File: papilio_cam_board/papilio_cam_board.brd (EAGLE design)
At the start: 68.6 x 68.6 mm, 23 parts, among them U2 V_REG_317SMD

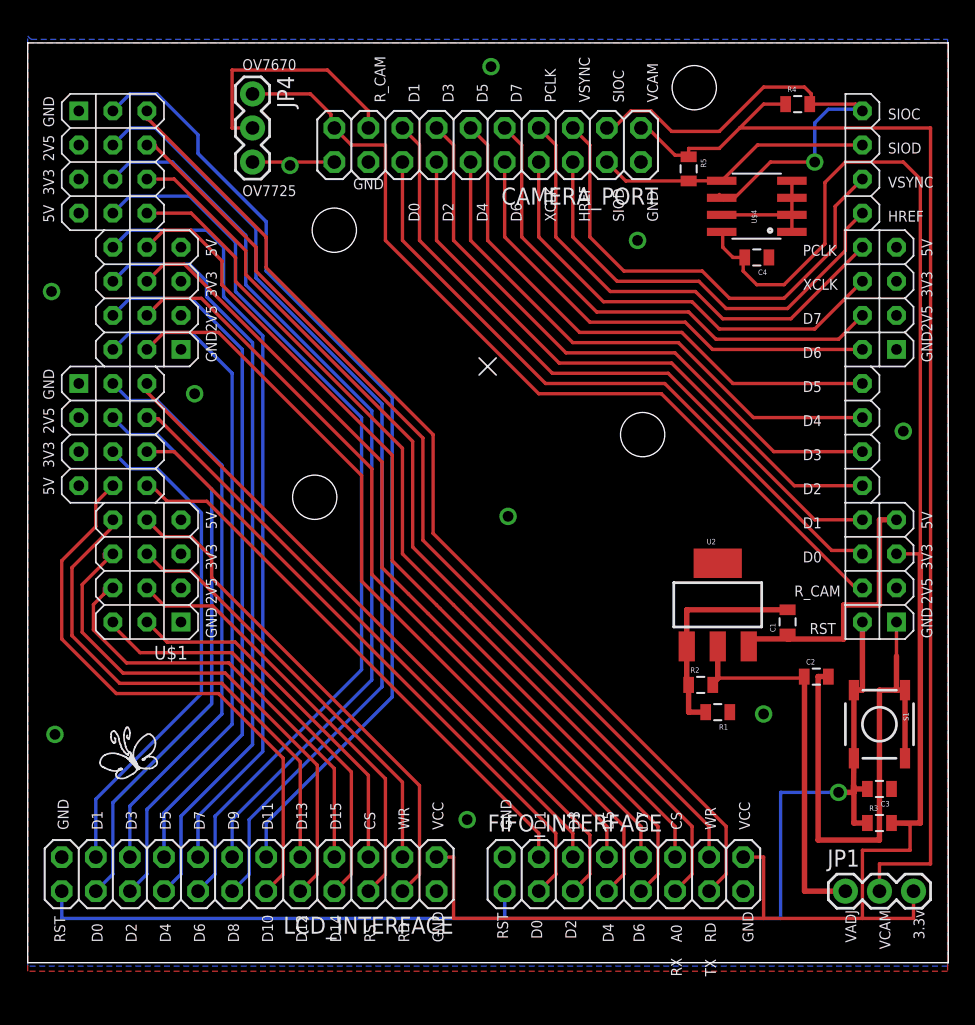
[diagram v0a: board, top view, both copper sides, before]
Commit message: modifying design
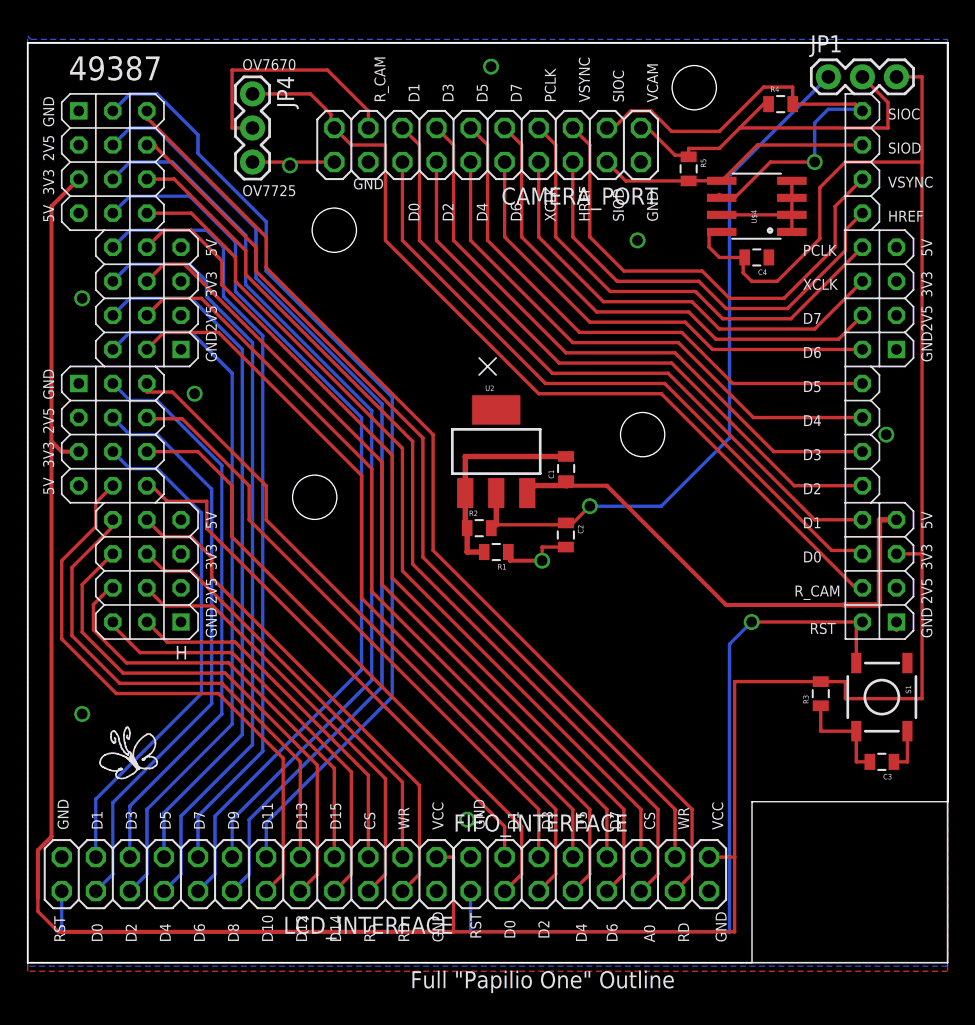
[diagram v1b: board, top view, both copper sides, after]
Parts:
- moved JP1 60.7 mm to (59.7, 66.0)
- moved C2 21.4 mm to (40.1, 31.9), turned to 270 degrees
- moved R1 20.4 mm to (34.9, 30.6)
- moved R2 20.2 mm to (33.7, 32.4)
- moved C1 20.1 mm to (40.1, 36.8)
- moved U2 20.1 mm to (34.9, 38.1)
- moved R3 10.6 mm to (59.1, 20.1), turned to 90 degrees
- moved FIFO_INTERFACE 2.54 mm to (41.9, 6.60)
- moved C3 2.03 mm to (63.7, 15.0)
- moved S1 2.03 mm to (63.7, 19.8)
- moved R4 1.27 mm to (56.1, 64.0)
- renumbered U$1 to H
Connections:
- new net N$3: C3.2, R3.1, S1.4
- new net N$4: C3.1, S1.2
- net 3.3V: now also H.W2_3V3_2, H.W2_3V3_4
- net GND: no longer C3.1, S1.2
- net RESET: no longer C3.2, R3.1, S1.4
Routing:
- net 3.3V: track 137.1 -> 229.8 mm
- net VCAM: track 89.0 -> 28.4 mm
- net GND: track 55.9 -> 21.6 mm, vias 10 -> 9
- net VADJ: track 29.2 -> 53.3 mm, vias 0 -> 1
- net 5V: track 21.5 -> 39.3 mm
- net N$3: track 0.00 -> 7.84 mm
- net N$4: track 0.00 -> 3.29 mm
- net FIFO_D6: track 62.5 -> 61.3 mm
- net FIFO_D4: track 68.0 -> 67.0 mm
- net FIFO_D5: track 61.6 -> 60.6 mm
- net FIFO_D1: track 70.8 -> 69.8 mm
- net FIFO_D3: track 66.2 -> 65.2 mm
- net FIFO_D2: track 71.6 -> 70.6 mm
- net FIFO_D0: track 76.7 -> 75.6 mm
- net FIFO_WR: track 41.7 -> 40.7 mm
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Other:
- outline, holes or cut-outs redrawn
- board text added: "49387"
- board text removed: "3.3v"
- board text removed: "RX"
- board text removed: "TX"
- board text removed: "VADJ"
